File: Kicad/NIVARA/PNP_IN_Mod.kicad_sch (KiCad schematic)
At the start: 6 parts, among them U7 LTV-357TB, U8 LTV-357TB

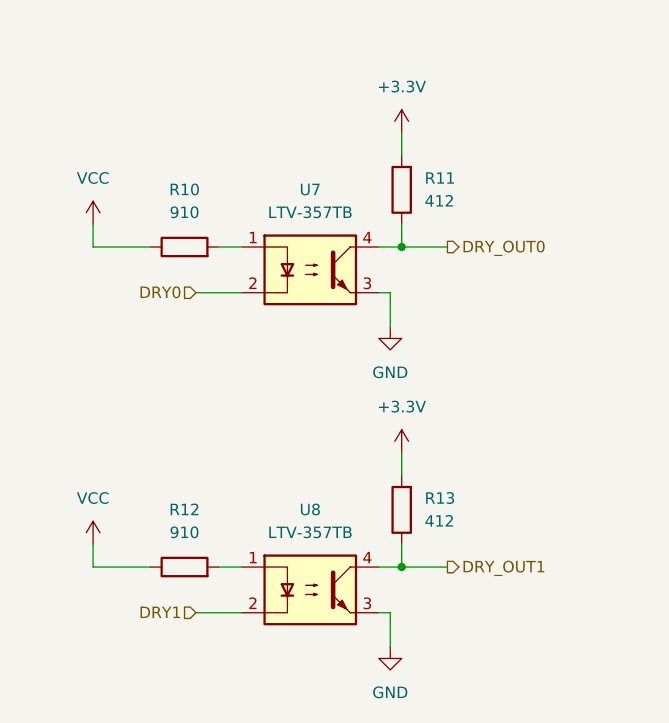
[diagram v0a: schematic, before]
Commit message: Rutinario
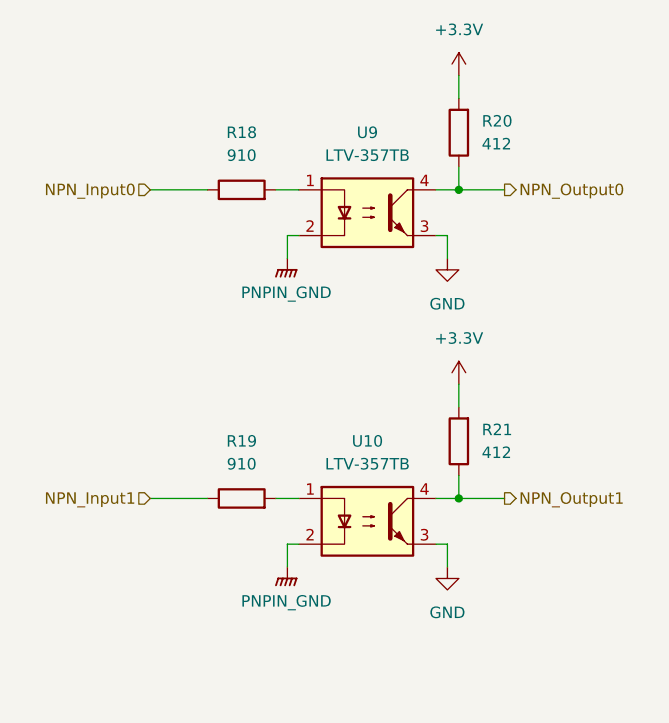
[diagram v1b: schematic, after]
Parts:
- removed R10, R12: 910, Resistor_SMD:R_0603_1608Metric, symbol Device:R
- removed R11, R13: 412, symbol Device:R
- removed U7, U8: LTV-357TB, Package_SO:SO-4_4.4x3.6mm_P2.54mm, symbol Isolator:LTV-357T
- added R18, R19: 910, Resistor_SMD:R_0603_1608Metric, symbol Device:R
- added R20, R21: 412, symbol Device:R
- added U10, U9: LTV-357TB, Package_SO:SO-4_4.4x3.6mm_P2.54mm, symbol Isolator:LTV-357T
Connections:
- net +3.3V: now also R20.2, R21.2
- net GND: now also U10.3, U9.3
- new net: R19.2, U10.1
- new net: R18.2, U9.1
- new net NPN_Input0: R18.1
- new net NPN_Input1: R19.1
- new net NPN_Output0: R20.1, U9.4
- new net NPN_Output1: R21.1, U10.4
- new net PNPIN_GND: U10.2, U9.2
